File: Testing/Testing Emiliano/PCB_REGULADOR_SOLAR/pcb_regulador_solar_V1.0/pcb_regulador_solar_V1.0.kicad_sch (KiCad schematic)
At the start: 187 parts, among them J1 Conn_01x03_Pin, J10 Conn_01x03_Pin, J2 Screw_Terminal_01x02, J3 INA219, J4 Conn_01x02_Pin, J5 Screw_Terminal_01x02, J6 USB_A, J7 Screw_Terminal_01x02, J8 Screw_Terminal_01x02, J9 INA219, Q1 BC557, Q10 2N3904, Q11 IRLIZ44N, Q12 IRF4905, Q13 2N7000, Q14 IRF4905, Q15 BC337, Q16 BC327, Q17 2N3904, Q18 2N3904, Q19 IRF4905, Q2 BC557, Q20 2N3904, Q21 2N3904, Q22 2N3904, Q23 BC557, Q24 BC557, Q3 2N3904, Q4 2N3904, Q5 2N3904, Q6 IRF4905, Q7 IRF4905, Q8 IRLIZ44N, Q9 BC557, SW1 RESET MANUAL, SW2 RESET MANUAL, SW3 RESET MANUAL, U1 PC817, U2 NE555P, U3 PC817, U4 LM358, U5 LM358, U6 PC817, U7 NE555P, U8 PC817

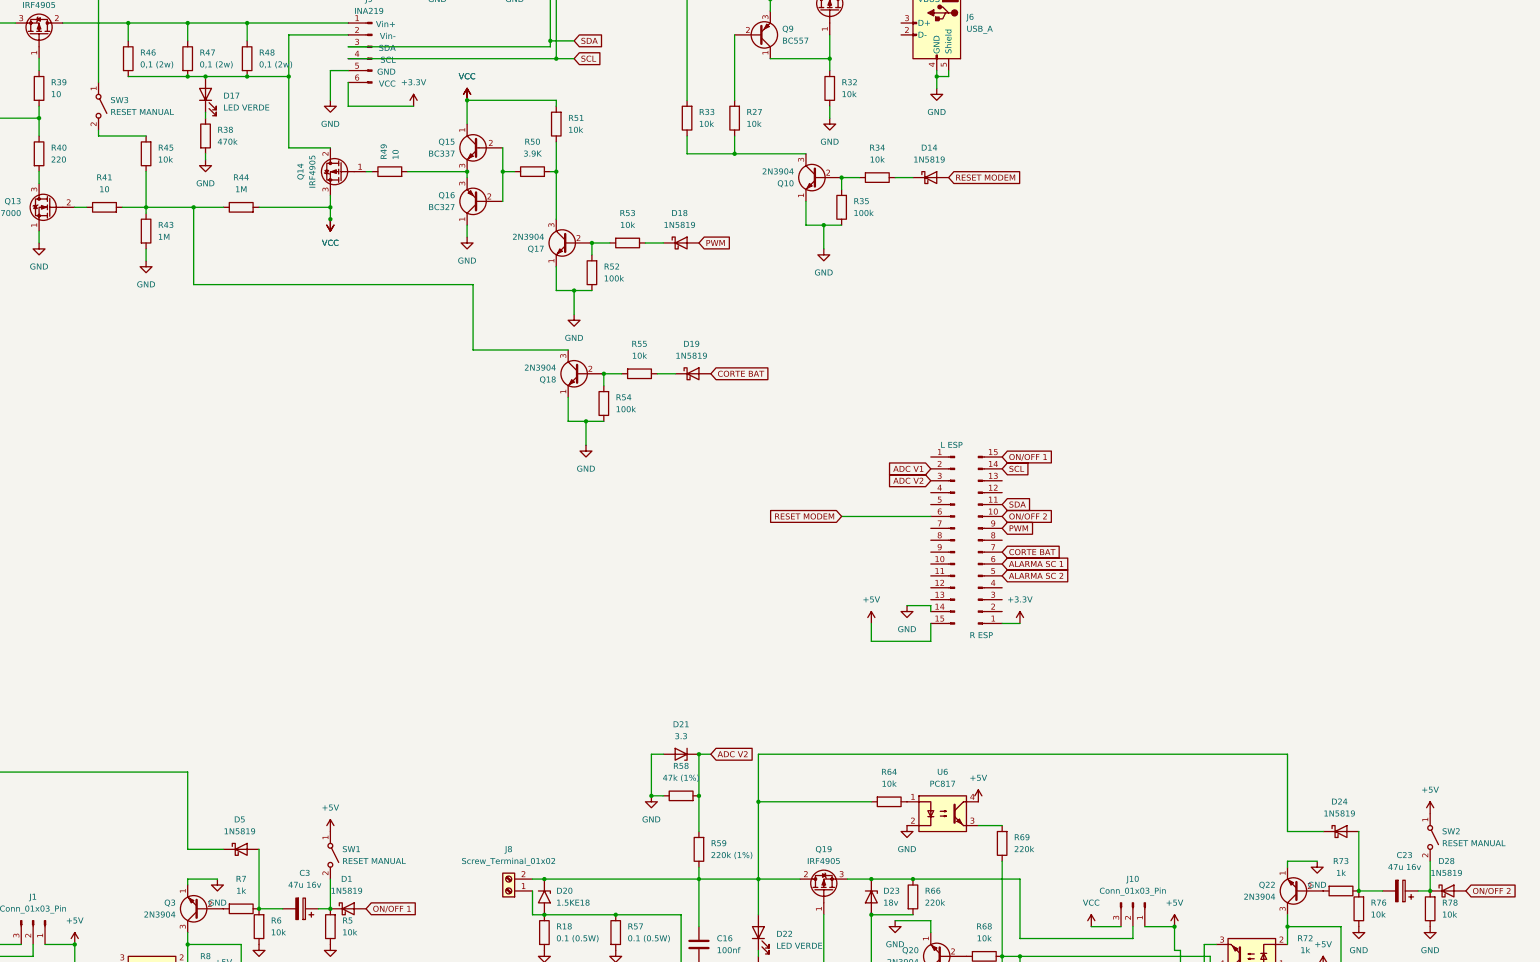
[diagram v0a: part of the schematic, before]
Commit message: pcb sOLAR
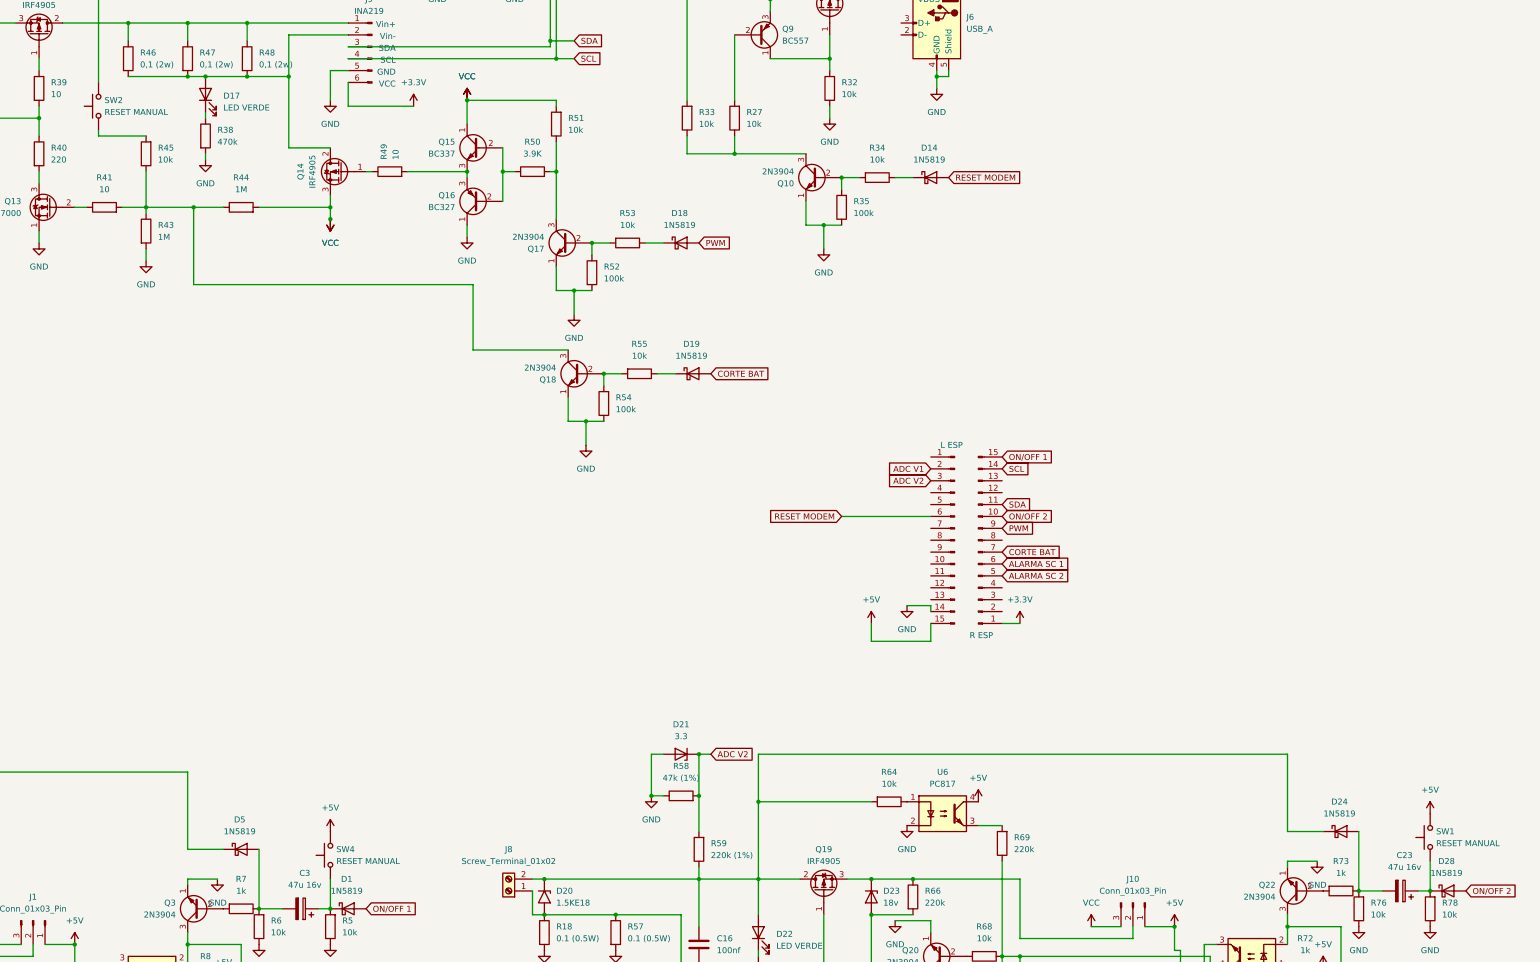
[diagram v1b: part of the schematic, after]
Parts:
- removed SW1, SW2, SW3: RESET MANUAL, symbol Switch:SW_SPST
- added SW1, SW2, SW4: RESET MANUAL, Button_Switch_SMD:SW_SPST_CK_RS282G05A3, symbol Switch:SW_Push
- D11, D17, D22, D27, D4, D7: footprint (none) -> LED_THT:LED_D3.0mm_IRBlack
- D13, D15, D16, D21, D23, D26, D3, D6, D8: footprint (none) -> Diode_THT:D_DO-35_SOD27_P7.62mm_Horizontal
- DCDC1, DCDC2, DCDC3, DCDC4, DCDC5, DCDC6, DCDC7, DCDC8: footprint (none) -> Connector_PinHeader_2.54mm:PinHeader_1x01_P2.54mm_Vertical
- F1, F2: footprint (none) -> Fuse:Fuseholder_Clip-5x20mm_Bel_FC-203-22_Lateral_P17.80x5.00mm_D1.17mm_Horizontal
- J1, J10: footprint (none) -> Connector_PinHeader_2.54mm:PinHeader_1x03_P2.54mm_Vertical
- J2, J5, J7, J8: footprint (none) -> TerminalBlock:TerminalBlock_bornier-3_P5.08mm
- J3, J9: footprint (none) -> Connector_PinSocket_2.54mm:PinSocket_1x06_P2.54mm_Vertical
- J4: footprint (none) -> Connector_PinHeader_2.54mm:PinHeader_1x02_P2.54mm_Vertical
- J6: footprint (none) -> Connector_USB:USB_A_Wuerth_614004134726_Horizontal
- LEFT_ESP1, RIGHT_ESP1: footprint (none) -> Connector_PinSocket_2.54mm:PinSocket_1x15_P2.54mm_Vertical
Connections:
- net +5V: now also SW1.2, SW4.2
- net at C23.1, D28.1 (K), R78.2: now also SW1.1
- net at C3.1, D1.1 (K), R5.2: now also SW4.1
- net at C13.1, C14.1, D15.1 (K)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: now also SW2.2
- net at R45.2: now also SW2.1

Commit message: Armado PCB
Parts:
- J2, J5, J7, J8: footprint TerminalBlock:TerminalBlock_bornier-3_P5.08mm -> TerminalBlock:TerminalBlock_bornier-2_P5.08mm
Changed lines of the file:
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@@
       (effects (font (size 1.27 1.27)))
     )
-    (property "Footprint" "TerminalBlock:TerminalBlock_bornier-3_P5.08mm" (at 281.94 260.35 0)
+    (property "Footprint" "TerminalBlock:TerminalBlock_bornier-2_P5.08mm" (at 281.94 260.35 0)
       (effects (font (size 1.27 1.27)) hide)
     )
@@
       (effects (font (size 1.27 1.27)))
     )
-    (property "Footprint" "TerminalBlock:TerminalBlock_bornier-3_P5.08mm" (at 73.66 34.29 0)
+    (property "Footprint" "TerminalBlock:TerminalBlock_bornier-2_P5.08mm" (at 73.66 34.29 0)
       (effects (font (size 1.27 1.27)) hide)
     )
@@
       (effects (font (size 1.27 1.27)))
     )
-    (property "Footprint" "TerminalBlock:TerminalBlock_bornier-3_P5.08mm" (at 72.39 77.47 0)
+    (property "Footprint" "TerminalBlock:TerminalBlock_bornier-2_P5.08mm" (at 72.39 77.47 0)
       (effects (font (size 1.27 1.27)) hide)
     )
@@
       (effects (font (size 1.27 1.27)))
     )
-    (property "Footprint" "TerminalBlock:TerminalBlock_bornier-3_P5.08mm" (at 46.99 264.16 0)
-      (effects (font (size 1.27 1.27)) hide)
-    )
+    (property "Footprint" "TerminalBlock:TerminalBlock_bornier-2_P5.08mm" (at 46.99 264.16 0)
+      (effects (font (size 1.27 1.27)) hide)
+    )

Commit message: actualizacion pcb_regulador_solar
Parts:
- removed C18, C21: 100nf, Capacitor_THT:C_Axial_L5.1mm_D3.1mm_P7.50mm_Horizontal, symbol Device:C
- removed C19, C20, C6: 10nf, Capacitor_THT:C_Axial_L5.1mm_D3.1mm_P7.50mm_Horizontal, symbol Device:C
- removed C22: 22u 25v, Capacitor_THT:C_Radial_D5.0mm_H11.0mm_P2.00mm, symbol Device:C_Polarized
- removed C23: 47u 16v, Capacitor_THT:C_Radial_D5.0mm_H11.0mm_P2.00mm, symbol Device:C_Polarized
- removed D13, D15, D16, D23, D6: 18v, Diode_THT:D_DO-35_SOD27_P7.62mm_Horizontal, symbol Device:D_Zener
- removed D17, D22: LED VERDE, LED_THT:LED_D3.0mm_IRBlack, symbol Device:LED
- removed D19, D2, D25, D28: 1N5819, Diode_THT:D_DO-41_SOD81_P10.16mm_Horizontal, symbol Diode:1N5819
- removed D20: 1.5KE18, Diode_THT:D_DO-201AE_P15.24mm_Horizontal, symbol Diode:1.5KExxA
- removed D21, D26, D3, D8: 3.3, Diode_THT:D_DO-35_SOD27_P7.62mm_Horizontal, symbol Device:D_Zener
- removed D27: LED ROJO, LED_THT:LED_D3.0mm_IRBlack, symbol Device:LED
- removed D9: 1N5822, Diode_THT:D_DO-201AD_P15.24mm_Horizontal, symbol Diode:1N5822
- removed J10: Conn_01x03_Pin, Connector_PinHeader_2.54mm:PinHeader_1x03_P2.54mm_Vertical, symbol Connector:Conn_01x03_Pin
- removed J4: Conn_01x02_Pin, Connector_PinHeader_2.54mm:PinHeader_1x02_P2.54mm_Vertical, symbol Connector:Conn_01x02_Pin
- removed J8: Screw_Terminal_01x02, TerminalBlock:TerminalBlock_bornier-2_P5.08mm, symbol Connector:Screw_Terminal_01x02
- removed Q1, Q2, Q23, Q24: BC557, Package_TO_SOT_THT:TO-92_Inline, symbol Transistor_BJT:BC557
- removed Q10, Q17, Q18, Q20, Q21, Q22, Q3, Q4, Q5: 2N3904, Package_TO_SOT_THT:TO-92_Inline, symbol Transistor_BJT:2N3904
- removed Q13: 2N7000, Package_TO_SOT_THT:TO-92_Inline, symbol Transistor_FET:2N7000
- removed Q19: IRF4905, Package_TO_SOT_THT:TO-220-3_Vertical, symbol Transistor_FET:IRF4905
- removed R65: 220, Resistor_THT:R_Axial_DIN0207_L6.3mm_D2.5mm_P2.54mm_Vertical, symbol Device:R
- removed R66, R69, R71: 220k, Resistor_THT:R_Axial_DIN0207_L6.3mm_D2.5mm_P2.54mm_Vertical, symbol Device:R
- removed R67: 1M, Resistor_THT:R_Axial_DIN0207_L6.3mm_D2.5mm_P2.54mm_Vertical, symbol Device:R
- removed R68, R70, R74, R75, R76, R78: 10k, Resistor_THT:R_Axial_DIN0207_L6.3mm_D2.5mm_P2.54mm_Vertical, symbol Device:R
- removed R72, R73: 1k, Resistor_THT:R_Axial_DIN0207_L6.3mm_D2.5mm_P2.54mm_Vertical, symbol Device:R
- removed R77: 47k, Resistor_THT:R_Axial_DIN0207_L6.3mm_D2.5mm_P2.54mm_Vertical, symbol Device:R
- removed R79: 100k, Resistor_THT:R_Axial_DIN0207_L6.3mm_D2.5mm_P2.54mm_Vertical, symbol Device:R
- removed SW2: RESET MANUAL, Button_Switch_SMD:SW_SPST_CK_RS282G05A3, symbol Switch:SW_Push
- removed U3, U6, U8: PC817, Package_DIP:DIP-4_W7.62mm, symbol Isolator:PC817
- removed U4, U5: LM358, Package_DIP:DIP-8_W7.62mm, symbol Amplifier_Operational:LM358
- removed U7: NE555P, Package_DIP:DIP-8_W7.62mm, symbol Timer:NE555P
- added ACS1, ACS4: OUT, Connector_PinHeader_2.54mm:PinHeader_1x01_P2.54mm_Vertical, symbol Connector:Conn_01x01_Pin
- added ACS2, ACS712: IN-, Connector_PinHeader_2.54mm:PinHeader_1x01_P2.54mm_Vertical, symbol Connector:Conn_01x01_Pin
- added ACS3, ACS712: Vcc, Connector_PinHeader_2.54mm:PinHeader_1x01_P2.54mm_Vertical, symbol Connector:Conn_01x01_Pin
- added ACS5, ACS712: IN+, Connector_PinHeader_2.54mm:PinHeader_1x01_P2.54mm_Vertical, symbol Connector:Conn_01x01_Pin
- added ACS6, ACS712: GND, Connector_PinHeader_2.54mm:PinHeader_1x01_P2.54mm_Vertical, symbol Connector:Conn_01x01_Pin
- added C18: 22u 16v, Capacitor_THT:C_Radial_D5.0mm_H11.0mm_P2.00mm, symbol Device:C_Polarized
- added C19: 47u 16v, Capacitor_THT:C_Radial_D5.0mm_H11.0mm_P2.00mm, symbol Device:C_Polarized
- added C6: 1u 16V, Capacitor_THT:C_Radial_D5.0mm_H11.0mm_P2.00mm, symbol Device:C_Polarized
- added D13, D16, D17, D19, D20, D21, D29, D30, D33, D6, D8, D9: 1N4746A, Diode_THT:D_DO-41_SOD81_P10.16mm_Horizontal, symbol Diode:1N47xxA
- added D15, D3: LED VERDE, LED_THT:LED_D3.0mm_IRBlack, symbol Device:LED
- added D2: 1.5KE18, Diode_THT:D_DO-201AE_P15.24mm_Horizontal, symbol Diode:1.5KExxA
- added D22, D31, D32: 1N5819, Diode_THT:D_DO-41_SOD81_P10.16mm_Horizontal, symbol Diode:1N5819
- added D23: LED ROJO, LED_THT:LED_D3.0mm_IRBlack, symbol Device:LED
- added D34: LED AZUL, LED_THT:LED_D3.0mm_IRBlack, symbol Device:LED
- added J4: OUT 2, TerminalBlock:TerminalBlock_bornier-2_P5.08mm, symbol Connector:Screw_Terminal_01x02
- added Q1, Q10, Q13, Q17, Q18, Q19, Q2, Q4, Q5: BC546, Package_TO_SOT_THT:TO-92_Inline, symbol Transistor_BJT:BC546
- added Q3: IRF4905, Package_TO_SOT_THT:TO-220-3_Vertical, symbol Transistor_FET:IRF4905
- added R80: 100k, Resistor_THT:R_Axial_DIN0207_L6.3mm_D2.5mm_P2.54mm_Vertical, symbol Device:R
- added SENSOR_TEMP: Conn_01x03_Pin, Connector_PinHeader_2.54mm:PinHeader_1x03_P2.54mm_Vertical, symbol Connector:Conn_01x03_Pin
- added U3: NE555P, Package_DIP:DIP-8_W7.62mm, symbol Timer:NE555P
- added U4: PC817, Package_DIP:DIP-4_W7.62mm, symbol Isolator:PC817
- C11, C8: value 100nf -> 100n
- C13: value 100n -> 100nf
- C14: value 100u 25v -> 1u 16V
- C17: value 100nf -> 10nf
- C4: value 22u 25v -> 22u 16v
- C9: value 1000u 25v -> 470u 50v
- F1, F2: value Fuse 3A -> Fuse 10A
- J2: value Screw_Terminal_01x02 -> OUT 1
- Q11, Q8: value IRLIZ44N -> IRFZ44N
- R12, R30, R37: value 220 -> 220 (1W)
- R13: value 10 -> 1M
- R16: value 10k -> 3.9 k
- R17: value 470k -> 22k
- R18: value 0.1 (0.5W) -> 3.9 k
- R2: value 100k -> 15k
- R20: value 0.1 (0.5W) -> 47k (1%)
- R21: value 0.1 (0.5W) -> 240k (1%)
- R22: value 10k (1%) -> 1M
- R23: value 220k (1%) -> 220 (1W)
- R28: value 470k -> 220 (1W)
- R29: value 10 -> 3.9K
- R36, R41: value 10 -> 220k
- R38: value 470k -> 470
- R39: value 10 -> 470
- R40: value 220 -> 10k
- R42: value 1M -> 10k
- R44: value 1M -> 220k
- R49: value 10 -> 220 (1W)
- R54: value 100k -> 10k
- R55: value 10k -> 22k
- R56: value 220k (1%) -> 240k (1%)
- R57: value 0.1 (0.5W) -> 47k
- R58: value 47k (1%) -> 220k
- R59, R62: value 220k (1%) -> 10k
- R60: value 10k (1%) -> 15k
- R61: value 470k -> 1k
- R63: value 10 -> 10k
- R7: value 1k -> 10k
- SW1: value RESET MANUAL -> ON/OFF 2
- SW4: value RESET MANUAL -> ON/OFF 1
- renumbered J7 to IN_BAT, J5 to IN_PANEL
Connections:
- net +3.3V: now also D32.2 (A), SENSOR_TEMP.3 (Pin_3); no longer J3.6 (Pin_6), J9.6 (Pin_6)
- net +5V: now also C16.2, C8.1, R57.1, R58.2, R61.1, ACS3.1 (Pin_1), ACS712.1 (Pin_1), U3.4 (R), U3.8 (VCC); no longer C11.2, C17.2
- net ADC V1: now also C10.1, LEFT_ESP1.4 (Pin_4); no longer LEFT_ESP1.2 (Pin_2)
- net ADC V2: now also C11.1, LEFT_ESP1.5 (Pin_5), R20.2, R21.2; no longer LEFT_ESP1.3 (Pin_3), R58.2, R59.2
- net ALARMA SC 1: now also LEFT_ESP1.8 (Pin_8), R1.2; no longer RIGHT_ESP1.6 (Pin_6)
- net ALARMA SC 2: now also LEFT_ESP1.9 (Pin_9), R59.2, R60.2; no longer RIGHT_ESP1.5 (Pin_5)
- net GND: now also C11.2, C13.1, C15.2, C17.2, C8.2, D10.2 (A2), D12.2 (A2), J2.1 (Pin_1), R15.1, R16.2, R17.1, R20.1, R22.2, R29.1, R41.1, R55.1, R63.1, R64.1, ACS6.1 (Pin_1), ACS712.1 (Pin_1), C18.2, C6.2, D15.1 (K), D16.2 (A), D2.2 (A2), D29.2 (A), D33.2 (A), D34.1 (K), D9.2 (A), J4.1 (Pin_1), Q1.3 (E), Q10.3 (E), Q13.3 (E), Q17.3 (E), Q18.3 (E), Q19.3 (E), Q2.3 (E), Q4.3 (E), Q5.3 (E), R80.1, SENSOR_TEMP.1 (Pin_1), U3.1 (GND); no longer C11.1, C12.2, C13.2, C15.1, C17.1, C8.1, R17.2, R20.2, R21.2, R22.1, R28.2, R38.2, R43.2, R54.1, R57.2, R58.1, R61.2
- net ON/OFF 1: now also LEFT_ESP1.7 (Pin_7); no longer RIGHT_ESP1.15 (Pin_15)
- net ON/OFF 2: now also D24.2 (A), LEFT_ESP1.10 (Pin_10); no longer RIGHT_ESP1.10 (Pin_10)
- net PWM: now also LEFT_ESP1.13 (Pin_13); no longer RIGHT_ESP1.9 (Pin_9)
- net RESET MODEM: now also LEFT_ESP1.12 (Pin_12); no longer LEFT_ESP1.6 (Pin_6)
- net VCC: now also R44.1, D17.1 (K), D19.1 (K), D20.1 (K), D21.1 (K), Q3.3 (S); no longer C10.1, R44.2
- net at D4.1 (K): now also R1.1, U2.3 (Q)
- net at C5.2, D10.1 (A1), D7.2 (A)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: now also ACS712.1 (Pin_1); no longer D5.1 (K), Q6.2 (D), R16.2
- net at R50.2, R51.1: now also Q17.1 (C)
- net at J9.1 (Pin_1), R46.1, R47.1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: now also F2.2, R37.2; no longer Q12.2 (D)
- net at R27.1, R33.1: now also Q10.1 (C)
- net at D7.1 (K): now also R16.1; no longer R17.1
- net at R30.1: now also Q8.1 (G), D29.1 (K), D9.1 (K); no longer R29.2
- net at D11.2 (A), D12.1 (A1), DCDC8.1 (Pin_1)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: no longer C12.1
- net at R3.2: now also C7.1, R17.2, U2.6 (THR)
- net at C4.1, R9.1, U1.3: now also Q2.1 (C)
- net at R63.2: now also R62.1, C19.2, D22.2 (A)
- net at R24.1, U1.2, U2.2 (TR): now also C6.1, Q1.1 (C); no longer C8.2
- net at R55.2: now also C17.1, R42.2, U3.6 (THR); no longer R54.2
- net at R23.1: now also Q4.1 (C); no longer R22.2
- net at J1.2 (Pin_2), Q6.3 (S), R14.1: now also D6.1 (K), D8.1 (K)
- net at R12.2, R14.2: now also Q6.1 (G), D6.2 (A), D8.2 (A); no longer R13.2
- net at R11.1, U1.4, U2.7 (DIS): now also R10.1; no longer R10.2, R15.1
- net at Q11.1 (G): now also R37.1, D16.1 (K), D33.1 (K); no longer R36.1
- net at R36.2: now also Q12.1 (G), R28.1, D13.2 (A), D30.2 (A); no longer R37.1
- net at J3.1 (Pin_1), R25.1, R26.1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: now also Q12.3 (S), R36.1, D13.1 (K), D30.1 (K)
- net at R11.2: now also R13.2, R15.2, Q18.2 (B)
- net at R12.1: now also Q18.1 (C)
- net at R45.2: now also R41.2, R43.2, Q4.2 (B)
- net at R52.2, R53.2: now also Q17.2 (B)
- net at D24.1 (K), R64.2: now also SW1.1, C19.1; no longer C16.2, R59.1
- net at D11.1 (K): now also R29.2; no longer R28.1
- net at R34.2, R35.2: now also Q10.2 (B)
- net at IN_PANEL.1 (Pin_1), Q8.2 (D): now also C12.2; no longer D12.2 (A2)
- net at F1.1, IN_PANEL.2 (Pin_2): now also C12.1
- net at R62.2: now also Q19.2 (B)
- net at DCDC2.1 (Pin_1): now also Q12.2 (D)
- net at R7.2: now also Q1.2 (B)
- net LED_BAT: now reaches RIGHT_ESP1.3 (Pin_3)
- net LED_BAT: now also R38.2
- net at R39.1: now also D34.2 (A); no longer Q12.1 (G)
- net at R38.1: now also D15.2 (A)
- net at Q14.1 (G), R49.1: now also D17.2 (A), D19.2 (A)
- net at R13.1: now also D5.1 (K), Q6.2 (D), ACS712.1 (Pin_1); no longer Q6.1 (G)
- net at R40.2: now also Q13.2 (B), R80.2
- net TEMP: now reaches LEFT_ESP1.11 (Pin_11)
- net TEMP: now also SENSOR_TEMP.2 (Pin_2)
- net CORTE BAT: no longer names the net of RIGHT_ESP1.7 (Pin_7)
- new net: D32.1 (K), J3.6 (Pin_6), J9.6 (Pin_6)
- new net: D20.2 (A), D21.2 (A), Q3.1 (G), R23.2, R44.2
- new net: ACS4.1 (Pin_1), R42.1
- new net: D31.1 (K), R40.1
- new net: ACS5.1 (Pin_1), D22.1 (K), Q3.2 (D), R43.1
- new net: C14.1, Q19.1 (C), R22.1, U3.2 (TR), U4.2
- new net: C18.1, Q5.1 (C), R58.1, U4.3
- new net: Q5.2 (B), R54.2
- new net: R61.2, U4.1
- new net: D23.1 (K), R59.1, U3.3 (Q)
- new net: D23.2 (A), R57.2
- new net: Q2.2 (B), R10.2
- new net: ACS2.1 (Pin_1), C13.2, D2.1 (A1), D3.2 (A), J4.2 (Pin_2), R21.1
- new net: Q13.1 (C), R28.2
- new net: R45.1, R54.1, U3.7 (DIS), U4.4
- new net: C15.1, U3.5 (CV)
- new net: ACS1.1 (Pin_1), R3.1
- new net: D3.1 (K), R18.1
- new net CORTE_INPANEL: D31.2 (A), LEFT_ESP1.6 (Pin_6)
- new net LED_ESTADO: R39.2, RIGHT_ESP1.5 (Pin_5)
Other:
- note added: "3V3"
- note removed: "VCC"
- moved on the sheet: C1, C2, C3, C4, C5, C7, D1, D10, D11, D14, D18, D5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
